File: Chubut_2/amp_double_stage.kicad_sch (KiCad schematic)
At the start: 3 parts, among them J7 In, J8 Out

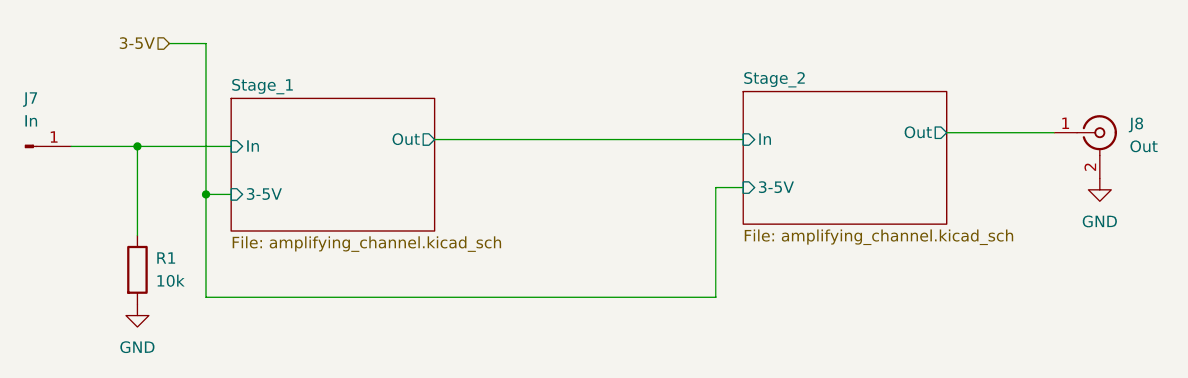
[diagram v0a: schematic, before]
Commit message: Schematic for the final version
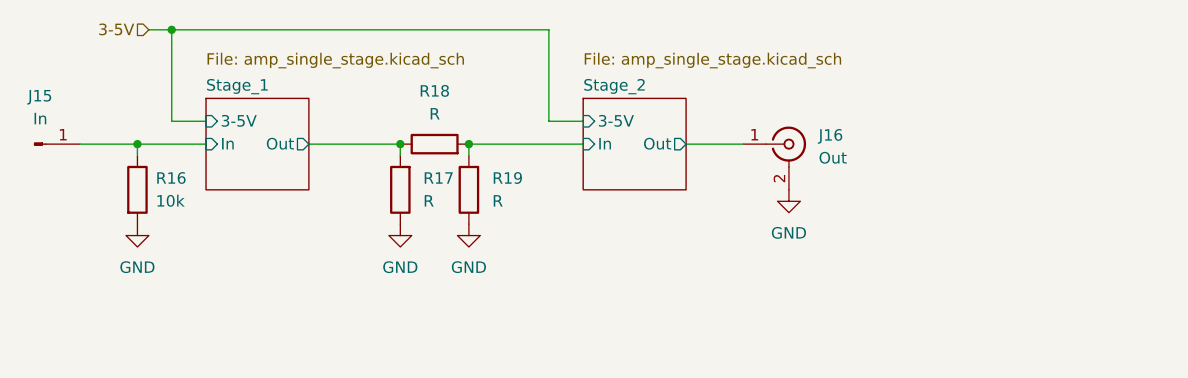
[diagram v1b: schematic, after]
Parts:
- added R17, R18, R19: R, Resistor_SMD:R_0402_1005Metric, symbol Device:R
- J16: renamed from J8; Digikey https://www.digikey.ch/short/n387fprw -> (none)
- renumbered J7 to J15, R1 to R16
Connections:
- net GND: now also R17.1, R19.1
- net Stage_1/Out: now also R17.2, R18.1
- new net Stage_2/In: R18.2, R19.2
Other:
- sheet Stage_1: file amplifying_channel.kicad_sch -> amp_single_stage.kicad_sch
- sheet Stage_2: file amplifying_channel.kicad_sch -> amp_single_stage.kicad_sch
- moved on the sheet: J15, J16, R16
